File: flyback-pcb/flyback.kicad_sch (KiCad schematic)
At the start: 14 parts, among them U1 MIN1072M-TL

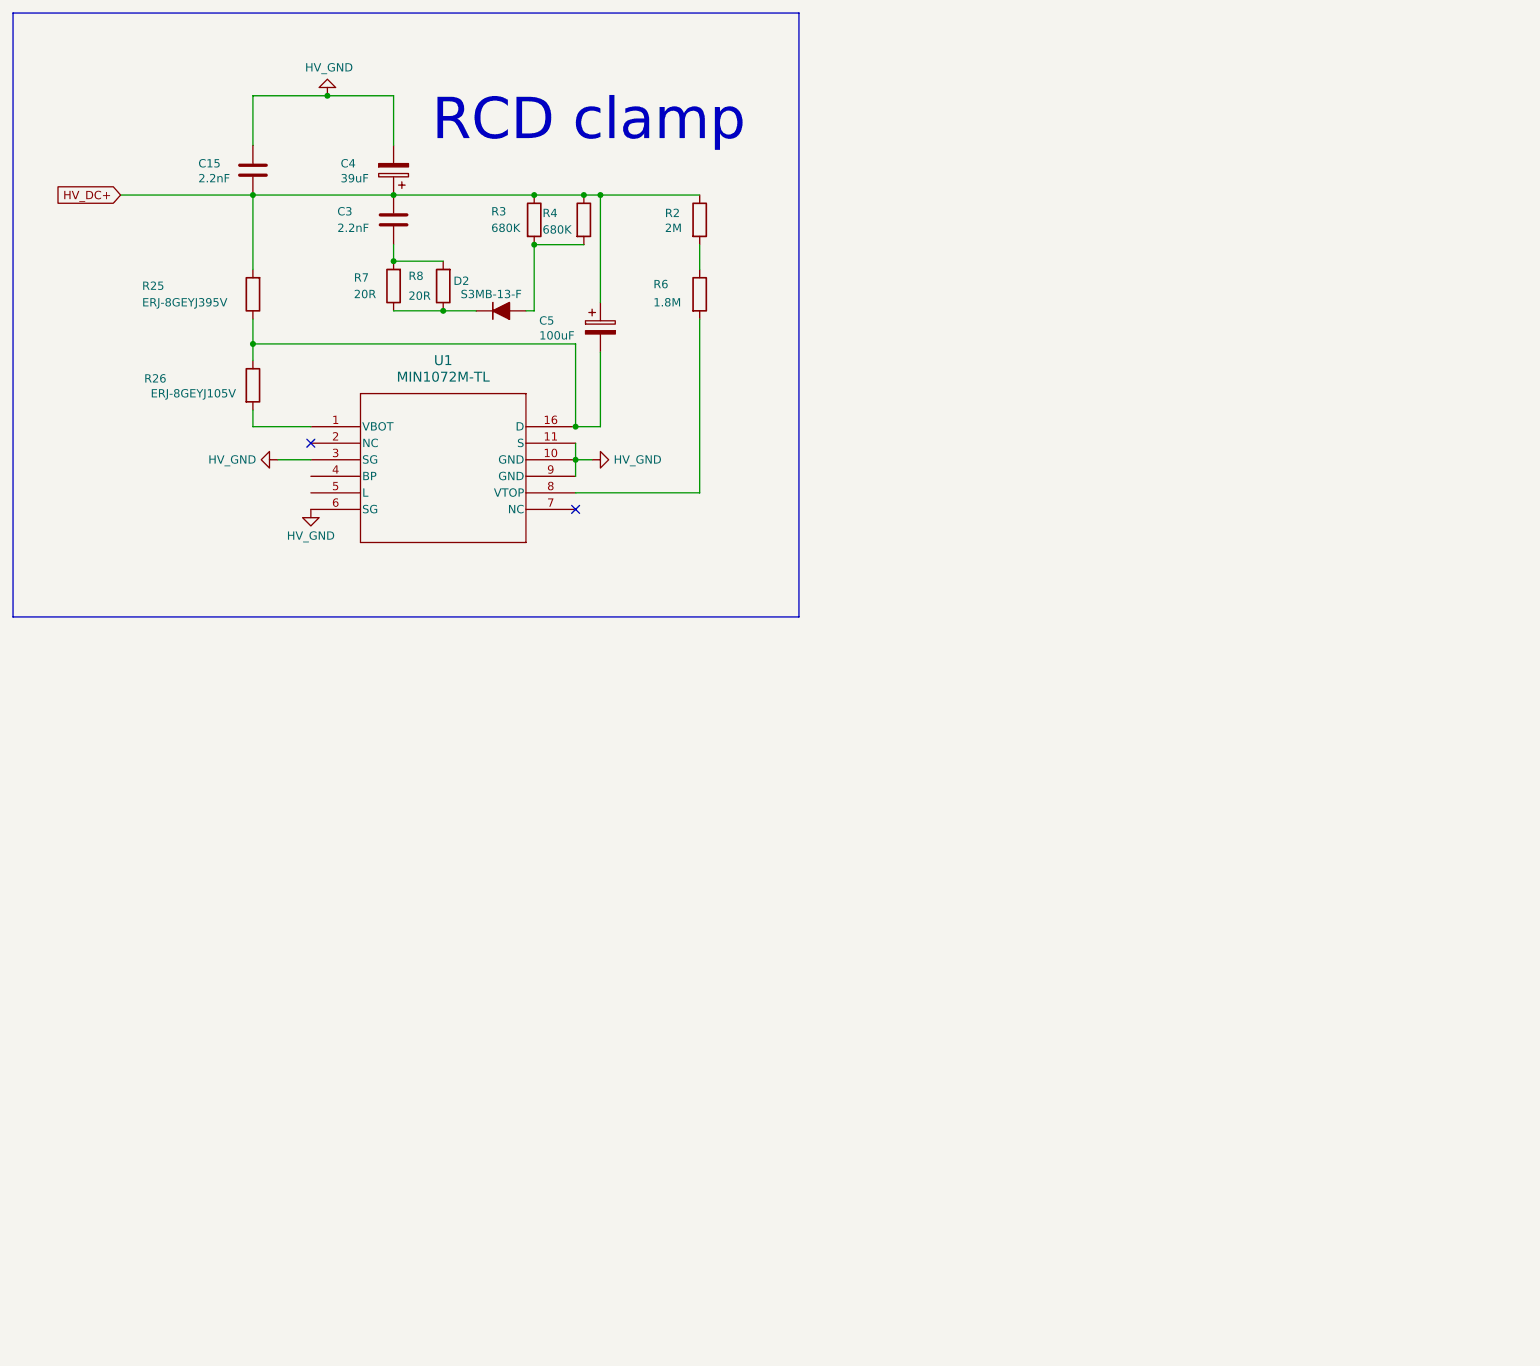
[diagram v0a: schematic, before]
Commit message: Done_Schematic_v0.1
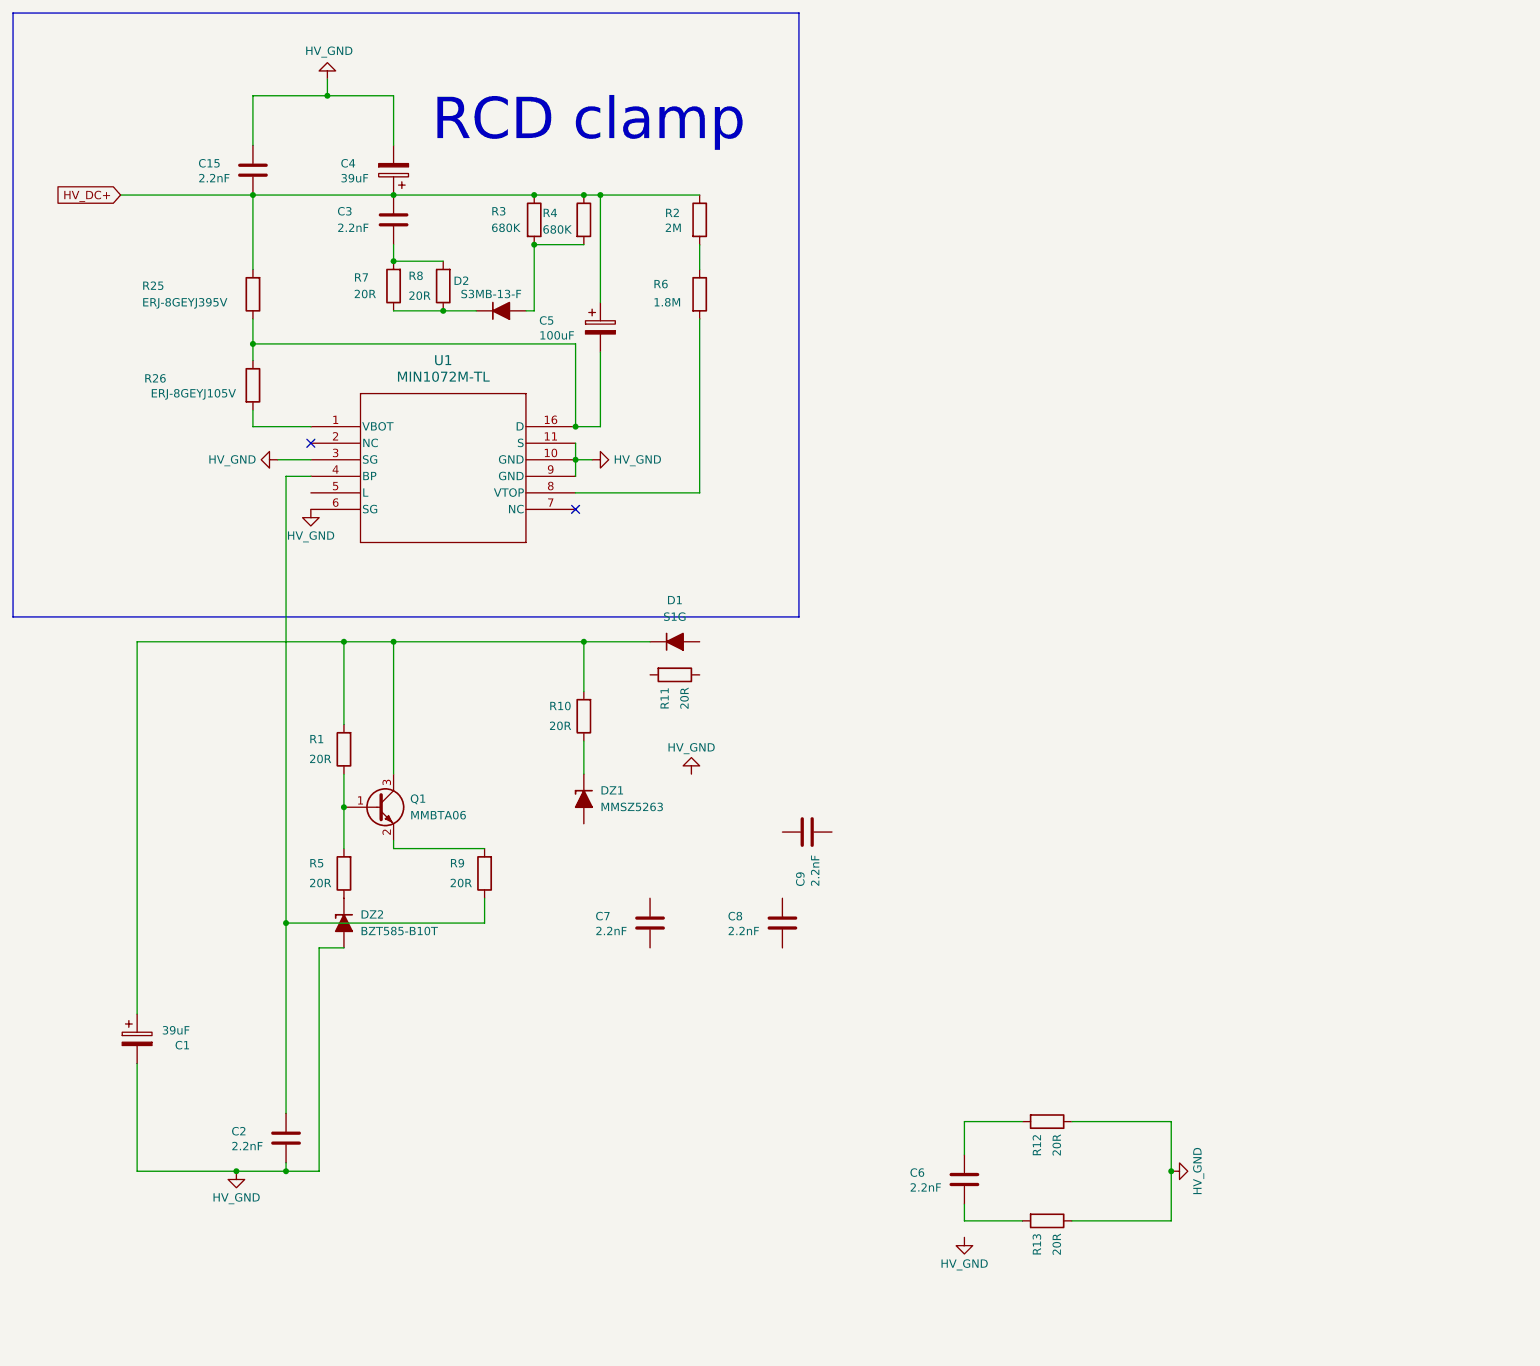
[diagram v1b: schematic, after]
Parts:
- added C1: 39uF, symbol Device:C_Polarized
- added C2, C6, C7, C8, C9: 2.2nF, symbol Device:C
- added D1: S1G, PCM_Diode_SMD_AKL:D_SMA, symbol emc_flyback_pcb:S1G
- added DZ1: MMSZ5263, PCM_Diode_SMD_AKL:D_SOD-123, symbol emc_flyback_pcb:MMSZ5263
- added DZ2: BZT585-B10T, PCM_Diode_SMD_AKL:D_SOD-523, symbol emc_flyback_pcb:BZT585-B10T
- added Q1: MMBTA06, Package_TO_SOT_SMD:SOT-23, symbol emc_flyback_pcb:MMBTA06
- added R1, R10, R11, R12, R13, R5, R9: 20R, symbol Device:R
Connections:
- net HV_GND: now also C1.2, C2.2, DZ2.2 (A), R12.1, R13.1
- net at U1.4 (BP): now also C2.1, R9.1
- new net: C1.1, D1.1 (K), Q1.3 (C), R1.2, R10.2
- new net: Q1.2 (E), R9.2
- new net: C6.2, R13.2
- new net: DZ2.1 (K), R5.1
- new net: Q1.1 (B), R1.1, R5.2
- new net: C6.1, R12.2
- new net: DZ1.1 (K), R10.1

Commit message: Scematic_V.2.0
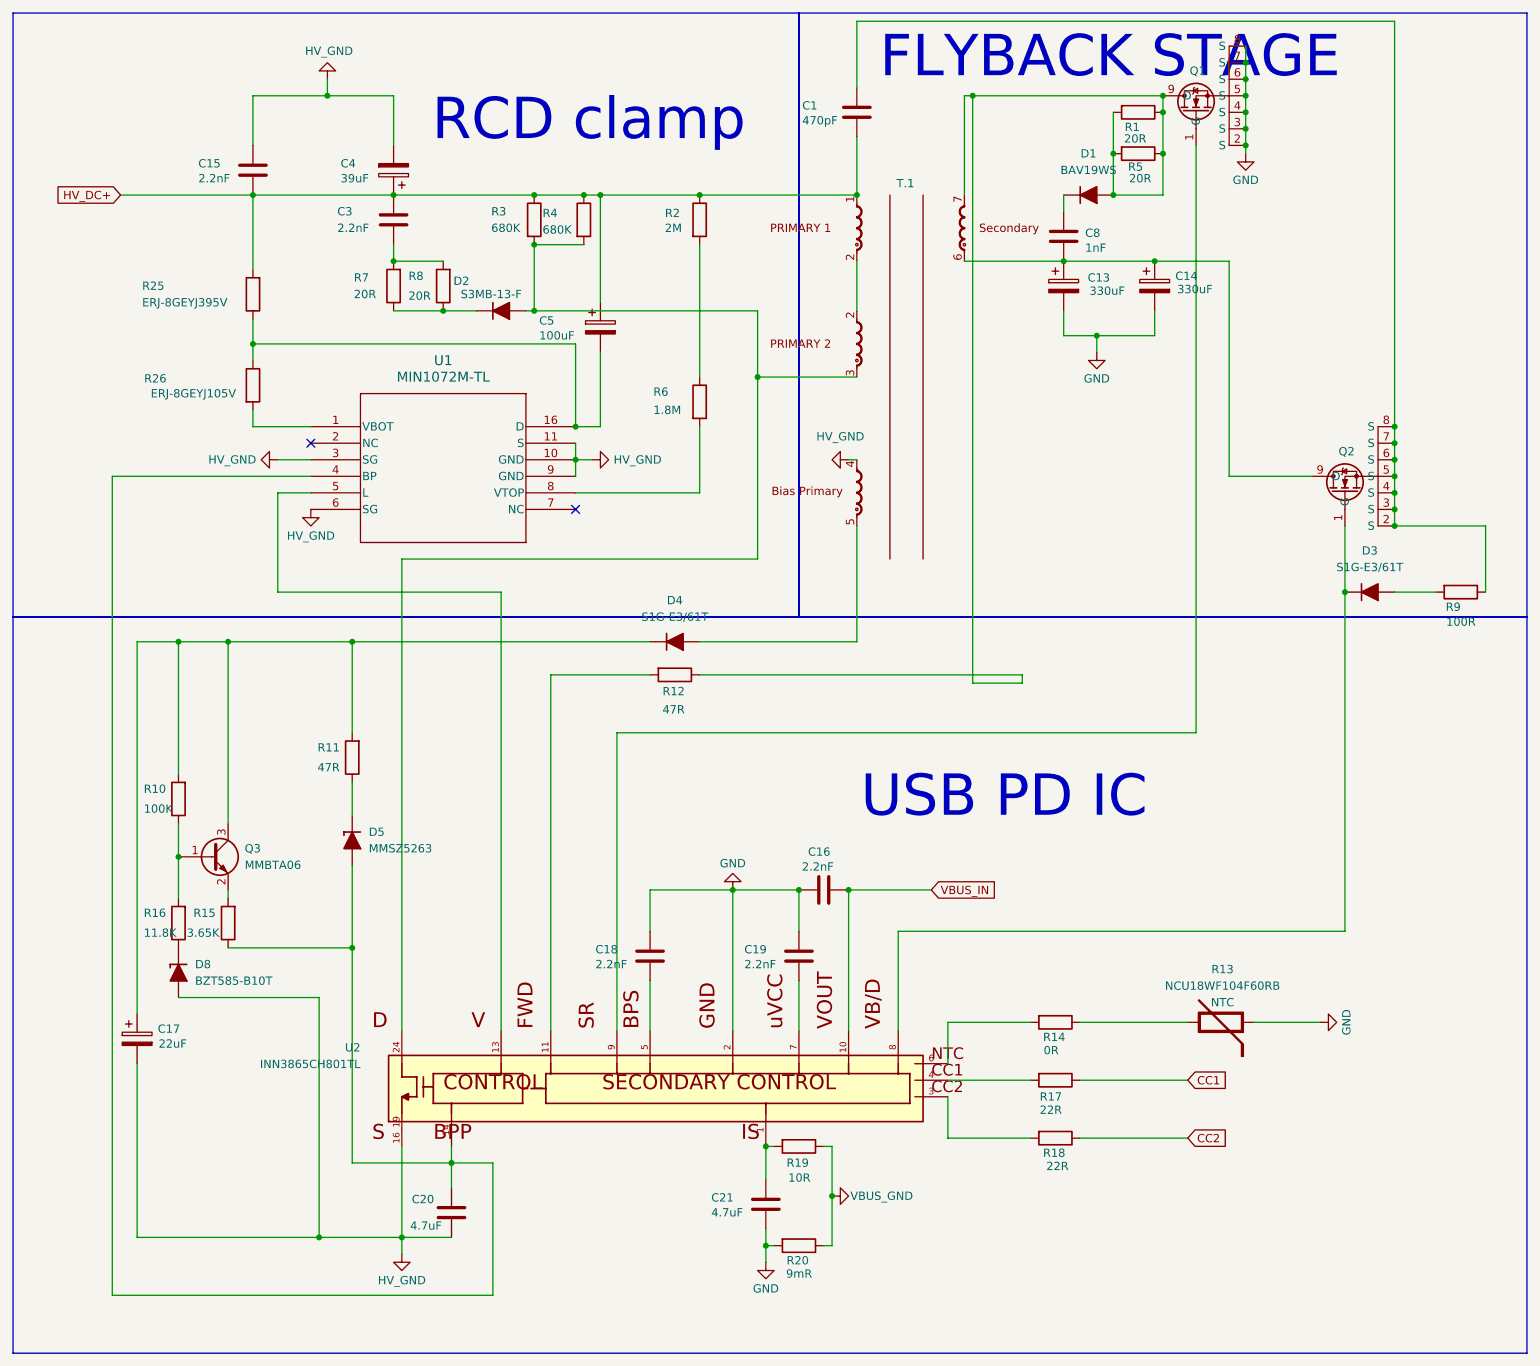
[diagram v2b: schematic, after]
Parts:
- removed U1: MIN1072M-TL, MINSOP-16A_PWI, symbol min1072m-tl:MIN1072M-TL
- added C1: 470pF, Capacitor_SMD:C_0603_1608Metric, symbol Device:C
- added C13, C14: 330uF, Capacitor_SMD:C_0603_1608Metric, symbol Device:C_Polarized
- added C8: 1nF, Capacitor_SMD:C_0603_1608Metric, symbol Device:C
- added D1: BAV19WS, Diode_SMD:D_SOD-323, symbol emc_flyback_pcb:BAV19WS
- added D3: S1G-E3/61T, Diode_SMD:D_SMA, symbol emc_flyback_pcb:S1G
- added Q1, Q2: ~, emc_flyback_pcb:H-PSOF8L-11.68X9.80_1, symbol emc_flyback_pcb:FDBL86210-F085
- added R1, R5: 20R, Resistor_SMD:R_0603_1608Metric, symbol Device:R
- added R13: NCU18WF104F60RB, Resistor_SMD:R_0603_1608Metric, symbol emc_flyback_pcb:NCU18WF104F60RB
- added R14: 0R, Resistor_SMD:R_0603_1608Metric, symbol Device:R
- added R15: 3.65K, Resistor_SMD:R_0603_1608Metric, symbol Device:R
- added R17, R18: 22R, Resistor_SMD:R_0603_1608Metric, symbol Device:R
- added T.1: ~, symbol emc_flyback_pcb:PQ3220
- added U1: MIN1072M-TL, emc_flyback_pcb:MINSOP-16A_PWI, symbol emc_flyback_pcb:MIN1072M-TL
- added U2: INN3865CH801TL, emc_flyback_pcb:IC_INN3865CH801TL, symbol emc_flyback_pcb:INN3865CH801TL
- C15, C3, C4, C5: footprint (none) -> Capacitor_SMD:C_0603_1608Metric
- C16: renamed from C9; footprint (none) -> Capacitor_SMD:C_0603_1608Metric
- C17: renamed from C1; value 39uF -> 22uF; footprint (none) -> Capacitor_SMD:C_0603_1608Metric
- C18: renamed from C7; footprint (none) -> Capacitor_SMD:C_0603_1608Metric
- C19: renamed from C8; footprint (none) -> Capacitor_SMD:C_0603_1608Metric
- C20: renamed from C2; value 2.2nF -> 4.7uF; footprint (none) -> Capacitor_SMD:C_0603_1608Metric
- C21: renamed from C6; value 2.2nF -> 4.7uF; footprint (none) -> Capacitor_SMD:C_0603_1608Metric
- D2: footprint PCM_Diode_SMD_AKL:D_SMBFL -> PCM_Diode_SMD_Handsoldering_AKL:D_SMBFL
- D4: renamed from D1; value S1G -> S1G-E3/61T; footprint PCM_Diode_SMD_AKL:D_SMA -> Diode_SMD:D_SMA
- D5: renamed from DZ1; footprint PCM_Diode_SMD_AKL:D_SOD-123 -> Diode_SMD:D_SOD-123
- D8: renamed from DZ2; footprint PCM_Diode_SMD_AKL:D_SOD-523 -> Diode_SMD:D_SOD-523
- R10: renamed from R1; value 20R -> 100K; footprint (none) -> Resistor_SMD:R_0603_1608Metric
- R11: renamed from R10; value 20R -> 47R; footprint (none) -> Resistor_SMD:R_0603_1608Metric
- R12: renamed from R11; value 20R -> 47R; footprint (none) -> Resistor_SMD:R_0603_1608Metric
- R16: renamed from R5; value 20R -> 11.8K; footprint (none) -> Resistor_SMD:R_0603_1608Metric
- R19: renamed from R12; value 20R -> 10R; footprint (none) -> Resistor_SMD:R_0603_1608Metric
- R2, R3, R4, R6, R7, R8: footprint (none) -> Resistor_SMD:R_0603_1608Metric
- R20: renamed from R13; value 20R -> 9mR; footprint (none) -> Resistor_SMD:R_0603_1608Metric
- R25, R26: footprint (none) -> Resistor_SMD:R_1206_3216Metric
- R9: value 20R -> 100R; footprint (none) -> Resistor_SMD:R_0603_1608Metric
- renumbered Q1 to Q3
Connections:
- net HV_DC+: now also C1.2, T.1.1
- net HV_GND: now also T.1.4, U1.10 (GND), U1.11 (S), U1.3 (SG), U1.6 (SG), U1.9 (GND), U2.16_19; no longer R19.1, R20.1
- net at D4.2 (A): now also T.1.5
- net at C5.2, R25.1, R26.1: now also U1.16 (D)
- net at D2.2 (A), R3.2, R4.2: now also T.1.3, U2.24
- net at C20.1: now also D5.2 (A), R15.1, U1.4 (BP), U2.14; no longer R9.1
- net at Q3.2 (E): now also R15.2; no longer R9.2
- net GND: now reaches C21.2, R20.2
- net GND: now also C16.1, C18.1, C19.1, C13.2, C14.2, Q1.2 (S), Q1.3 (S), Q1.4 (S), Q1.5 (S), Q1.6 (S), Q1.7 (S), Q1.8 (S), R13.2 (-), U2.2
- net at C18.2: now also U2.5
- net at R26.2: now also U1.1 (VBOT)
- net at R6.2: now also U1.8 (VTOP)
- net VBUS_IN: now reaches C16.2
- net VBUS_IN: now also U2.10
- net at R12.1: now also D1.2 (A), Q1.9 (D), R1.1, R1.2, R5.1, R5.2, T.1.7
- net at R12.2: now also U2.11
- net at C19.2: now also U2.7
- net at C21.1, R19.2: now also U2.1
- new net: U1.5 (L), U2.13
- new net: C1.1, Q2.2 (S), Q2.3 (S), Q2.4 (S), Q2.5 (S), Q2.6 (S), Q2.7 (S), Q2.8 (S), R9.1
- new net: C8.1, D1.1 (K)
- new net: R13.1 (+), R14.1
- new net: R14.2, U2.6
- new net: C13.1, C14.1, C8.2, Q2.9 (D), T.1.6
- new net: D3.1 (K), Q2.1 (G), U2.8
- new net: D3.2 (A), R9.2
- new net: Q1.1 (G), U2.9
- new net: R17.2, U2.4
- new net: R18.2, U2.3
- new net CC1: R17.1
- new net CC2: R18.1
- new net VBUS_GND: R19.1, R20.1
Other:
- note added: "FLYBACK STAGE"
- note added: "USB PD IC"
- moved on the sheet: C16, C18, C19, C20, C21, D5, D8, Q3, R10, R11, R16, R19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
